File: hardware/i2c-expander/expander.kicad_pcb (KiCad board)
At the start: 2 copper layers, 57.1 x 45.7 mm, 17 parts, among them IC1 MCP23017, IC2 MCP23017, J1 CONN_01X04, J2 CONN_02X03, J3 CONN_02X03, J4 CONN_02X08, J5 CONN_02X03, J6 CONN_02X03, J7 CONN_02X08, J8 CONN_01X04

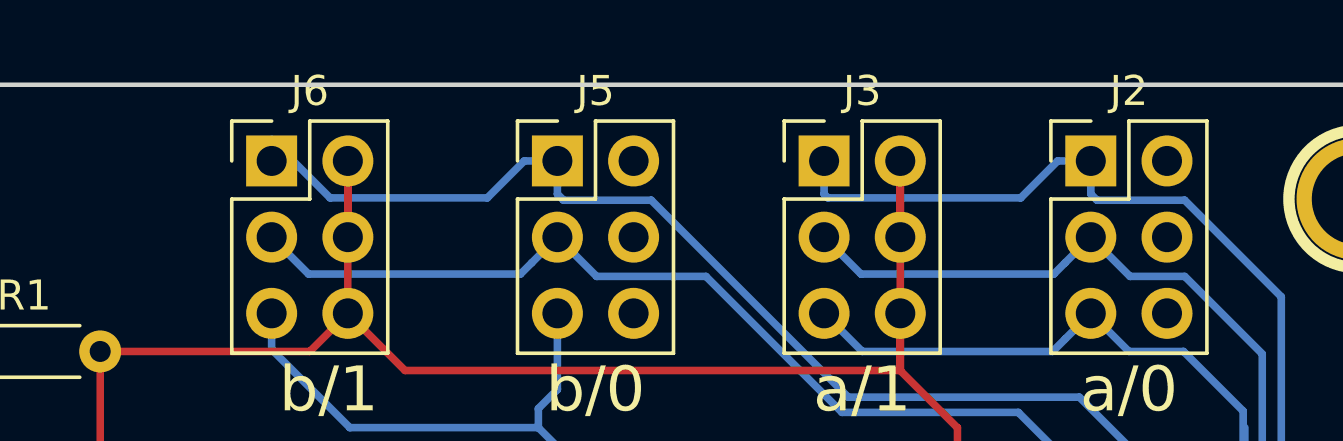
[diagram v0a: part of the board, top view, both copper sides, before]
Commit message: sent for production
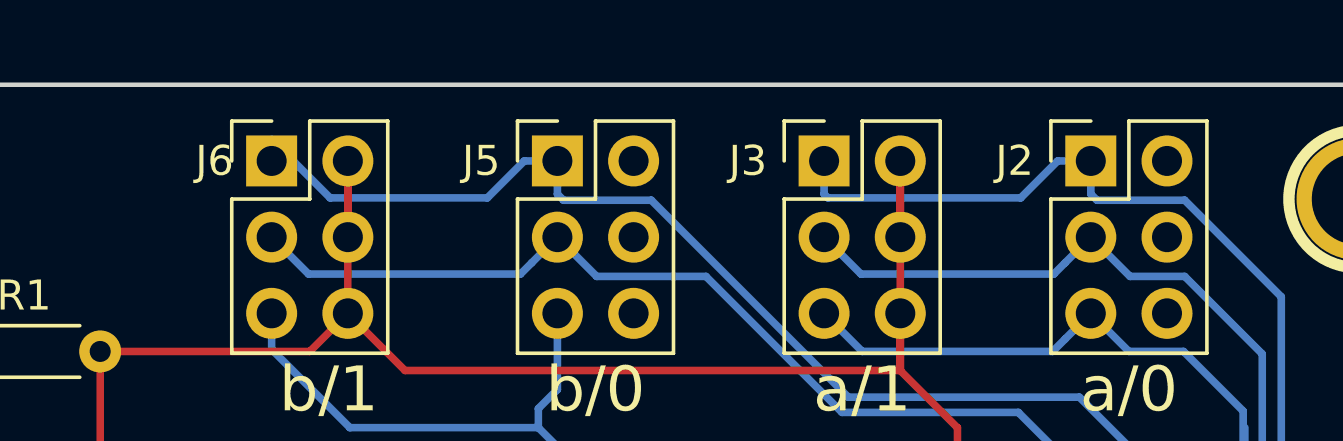
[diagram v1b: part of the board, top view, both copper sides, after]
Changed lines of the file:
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@@
 (kicad_pcb (version 4) (host pcbnew 4.0.6-e0-6349~53~ubuntu14.04.1)
   (general
-    (links 139)
-    (no_connects 52)
-    (area 173.914999 123.114999 231.215001 168.985001)
+    (links 75)
+    (no_connects 0)
+    (area 172.712667 122.8598 232.417334 169.552333)
     (thickness 1.6)
     (drawings 16)
@@
   (page A3)
   (layers
-    (0 F.Cu signal)
+    (0 F.Cu signal hide)
     (31 B.Cu signal)
     (32 B.Adhes user)
@@
     (visible_elements FFFFEFBF)
     (pcbplotparams
-      (layerselection 0x00030_80000001)
+      (layerselection 0x01fff_80000001)
       (usegerberextensions true)
       (excludeedgelayer true)
@@
       (outputformat 1)
       (mirror false)
-      (drillshape 1)
+      (drillshape 0)
       (scaleselection 1)
-      (outputdirectory svg/i2cexpander/))
+      (outputdirectory ../production/i2c-expander/))
   )
   (net 0 "")
@@
     (descr "Through hole straight pin header, 2x03, 2.54mm pitch, double rows")
     (tags "Through hole pin header THT 2x03 2.54mm double row")
-    (fp_text reference J2 (at 1.27 -2.33) (layer F.SilkS)
+    (fp_text reference J2 (at -2.54 0) (layer F.SilkS)
       (effects (font (size 1 1) (thickness 0.15)))
     )
@@
     (descr "Through hole straight pin header, 2x03, 2.54mm pitch, double rows")
     (tags "Through hole pin header THT 2x03 2.54mm double row")
-    (fp_text reference J3 (at 1.27 -2.33) (layer F.SilkS)
+    (fp_text reference J3 (at -2.54 0) (layer F.SilkS)
       (effects (font (size 1 1) (thickness 0.15)))
     )
@@
     (descr "Through hole straight pin header, 2x03, 2.54mm pitch, double rows")
     (tags "Through hole pin header THT 2x03 2.54mm double row")
-    (fp_text reference J5 (at 1.27 -2.33) (layer F.SilkS)
+    (fp_text reference J5 (at -2.54 0) (layer F.SilkS)
       (effects (font (size 1 1) (thickness 0.15)))
     )
@@
     (descr "Through hole straight pin header, 2x03, 2.54mm pitch, double rows")
     (tags "Through hole pin header THT 2x03 2.54mm double row")
-    (fp_text reference J6 (at 1.27 -2.33) (layer F.SilkS)
-      (effects (font (size 1 1) (thickness 0.15)))
-    )
+    (fp_text reference J6 (at -1.905 0) (layer F.SilkS)
+      (effects (font (size 1 1) (thickness 0.15)))
+    )
